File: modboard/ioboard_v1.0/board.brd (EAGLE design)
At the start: 50 x 42 mm, 20 parts, among them J2 POWER_JACKPTH

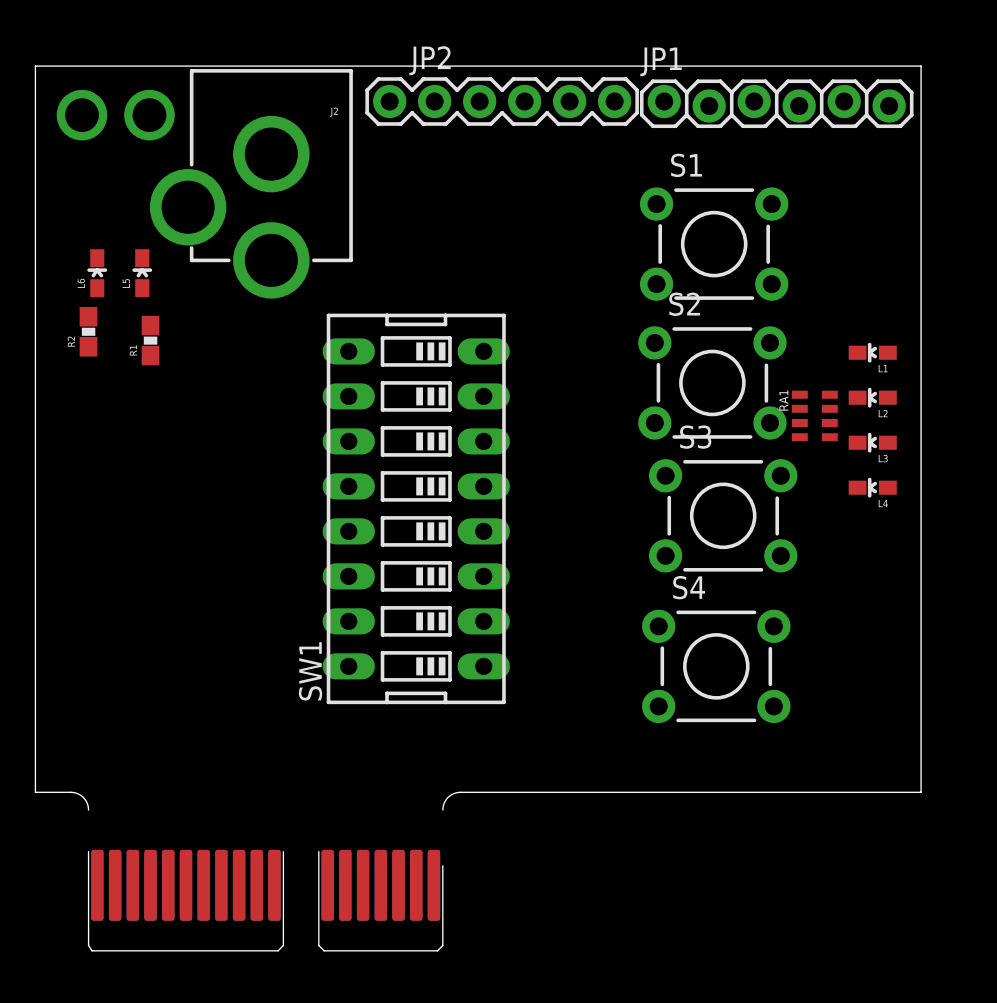
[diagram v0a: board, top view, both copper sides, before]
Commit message: finished the base modboards
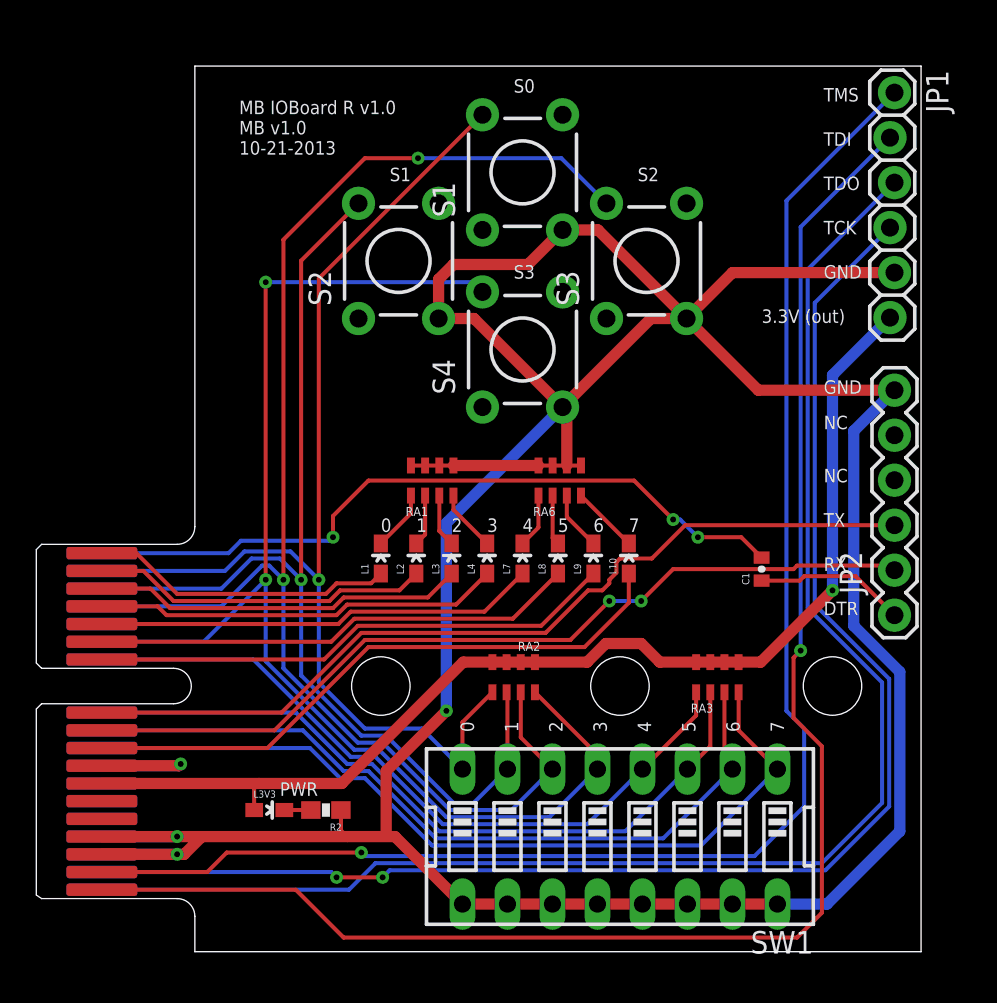
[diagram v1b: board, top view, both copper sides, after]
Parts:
- removed CONN1, CONN2: (no value), kmod-nonparts:HOLE_18AWG
- removed J2: POWER_JACKPTH, SparkFun-Connectors:POWER_JACK_PTH
- removed L5, L6: YLW, kmod-passives:0603_LED
- removed R1: 2.2k, kmod-passives:0603-RES
- added C1: 100nF, kmod-passives:0402-CAP
- added L10, L7, L8, L9: (no value), kmod-passives:0603_LED
- added L3V3: YLW, kmod-passives:0603_LED
- added RA2, RA3: 10k, kmod-passives:0603-ARV
- added RA6: 220, kmod-passives:0603-ARV
- moved JP2 40.7 mm to (48.5, 19.0), turned to 90 degrees
- moved R2 30.1 mm to (16.4, 8.00), turned to 180 degrees
- moved L1 30.1 mm to (19.5, 22.2), turned to 0 degrees
- moved L2 27.3 mm to (21.5, 22.2), turned to 0 degrees
- moved L3 24.7 mm to (23.5, 22.2), turned to 0 degrees
- moved L4 22.1 mm to (25.5, 22.2), turned to 0 degrees
- moved RA1 21.9 mm to (22.4, 26.6), turned to 0 degrees
- moved SW1 21.8 mm to (33.0, 6.50), turned to 180 degrees
- moved S4 21.0 mm to (27.5, 34.0), turned to 90 degrees
- moved S2 19.0 mm to (20.5, 39.0), turned to 90 degrees
- moved S3 15.0 mm to (34.5, 39.0), turned to 90 degrees
- moved U$1 14.8 mm to (4.50, 15.0), flipped to the bottom, turned to 90 degrees
- moved JP1 13.0 mm to (48.5, 48.5), turned to 270 degrees
- moved S1 11.6 mm to (27.5, 44.0), turned to 90 degrees
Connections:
- removed net 12V: CONN1.P$1, J2.GNDBREAK, L5.A, U$1.A8, U$1.B8
- removed net N$1: L5.C, R1.2
- removed net N$10: JP2.RXI
- removed net N$9: JP2.TXO
- new net A0: L4.A, U$1.A15
- new net A1: L3.A, U$1.A16
- new net A2: L2.A, U$1.A17
- new net A3: L1.A, U$1.A18
- new net B0: RA2.7, S3.2, SW1.6, U$1.B15
- new net B1: RA2.6, S2.2, SW1.7, U$1.B16
- new net B2: RA2.5, S1.2, SW1.8, U$1.B17
- new net B3: C1.2, U$1.B18
- new net C0: JP2.RXI, U$1.A10
- new net C1: JP2.TXO, U$1.A11
- new net C2: L9.A, U$1.A12
- new net C3: L8.A, U$1.A13
- new net D0: RA3.3, SW1.2, U$1.B10
- new net D1: RA3.2, SW1.3, U$1.B11
- new net D2: RA3.1, SW1.4, U$1.B12
- new net D3: RA2.8, S4.2, SW1.5, U$1.B13
- new net E0: L10.A, U$1.A9
- new net E1: RA3.4, SW1.1, U$1.B9
- new net E2: L7.A, U$1.A14
- new net E3: U$1.B14
- new net N$14: L7.C, RA6.1
- new net N$15: L8.C, RA6.2
- new net N$16: L9.C, RA6.3
- new net N$17: L10.C, RA6.4
- new net N$22: U$1.A8, U$1.B8
- net 3.3V: now also L3V3.A, RA2.1, RA2.2, RA2.3, RA2.4, RA3.5, RA3.6, RA3.7, RA3.8; no longer L6.A
- net GND: now also JP2.GND, RA6.5, RA6.6, RA6.7, RA6.8, SW1.10, SW1.11, SW1.12, SW1.13, SW1.14, SW1.15, SW1.16, SW1.9, U$1.B3; no longer CONN2.P$1, J2.PWR, R1.1, S1.4, S2.4, S3.4, S4.4, U$1.A2
- net N$11: now also C1.1
- net N$6: now also L3V3.C; no longer L6.C
- net TMS: now also U$1.A2
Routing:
- net GND: track 0.00 -> 196.5 mm, vias 0 -> 3
- net TDI: track 0.00 -> 89.0 mm, vias 0 -> 1
- net TDO: track 0.00 -> 84.9 mm
- net TMS: track 0.00 -> 84.6 mm, vias 0 -> 1
- net TCK: track 0.00 -> 82.6 mm, vias 0 -> 2
- net B0: track 0.00 -> 81.5 mm, vias 0 -> 2
- net D3: track 0.00 -> 73.9 mm, vias 0 -> 2
- net 3.3V: track 0.00 -> 65.0 mm, vias 0 -> 1
- net B2: track 0.00 -> 64.4 mm, vias 0 -> 1
- net B1: track 0.00 -> 60.2 mm, vias 0 -> 1
- net C1: track 0.00 -> 49.6 mm
- net C0: track 0.00 -> 48.7 mm, vias 0 -> 2
- net E1: track 0.00 -> 47.5 mm
- net D0: track 0.00 -> 44.3 mm
- net D1: track 0.00 -> 42.2 mm
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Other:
- board size 50 x 42 mm -> 42 x 50 mm
- board text added: "0"
- board text added: "1"
- board text added: "2"
- board text added: "3"
- board text added: "3.3V (out)"
- board text added: "4"
- board text added: "5"
- board text added: "6"
- board text added: "7"
- board text added: "DTR"
- board text added: "GND"
- board text added: "MB IOBoard R v1.0 MB v1.0 10-21-2013"
- board text added: "NC"
- board text added: "PWR"
- board text added: "RX"
- board text added: "S0"
- board text added: "S1"
- board text added: "S2"
- board text added: "S3"
- board text added: "TCK"
- board text added: "TDI"
- board text added: "TDO"
- board text added: "TMS"
- board text added: "TX"
